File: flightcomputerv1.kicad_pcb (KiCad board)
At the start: 2 copper layers, 190.5 x 101.6 mm, 3 parts, among them U1 Teensy4.1, U2 MS5607-02BA, U3 BMI088

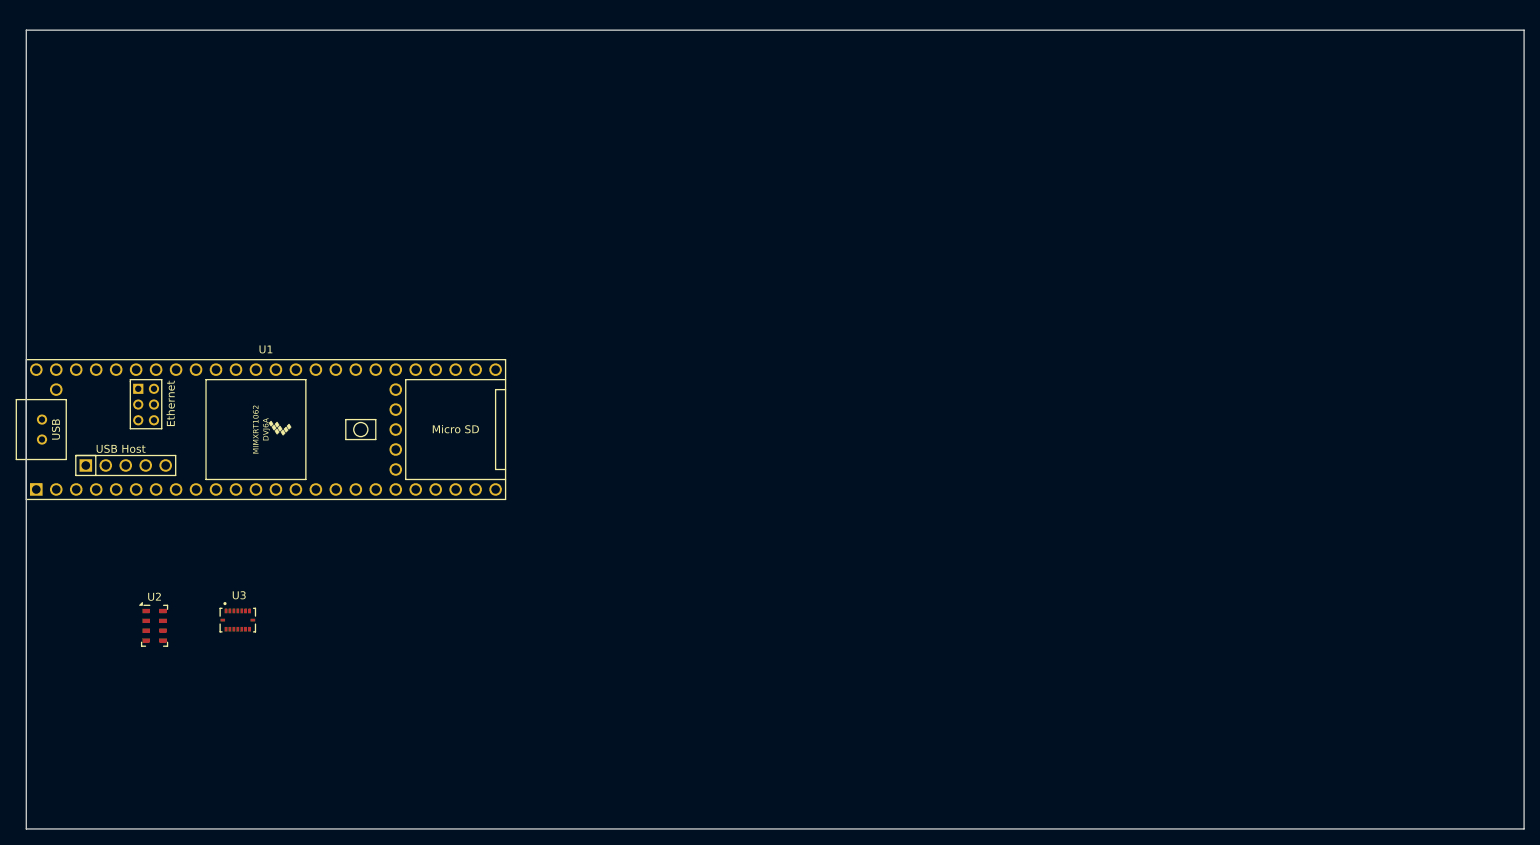
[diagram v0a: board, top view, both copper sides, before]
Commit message: started placement
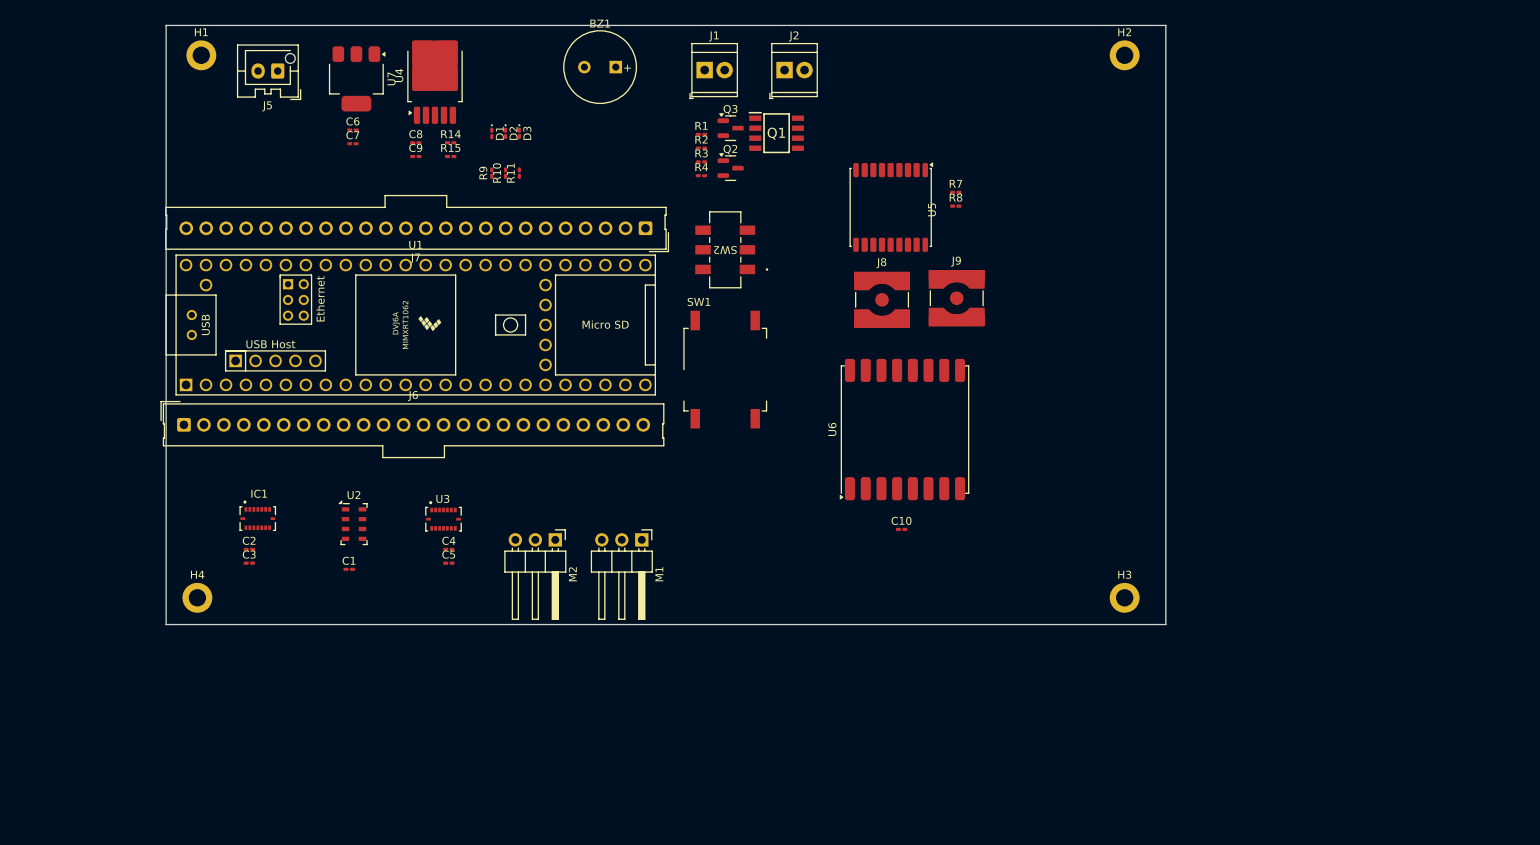
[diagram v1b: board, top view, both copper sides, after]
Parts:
- added BZ1: Buzzer, Buzzer_Beeper:MagneticBuzzer_PUI_AT-0927-TT-6-R, F.Cu at (108.0, 55.5)
- added C1: 0.1uF, Capacitor_SMD:C_0201_0603Metric_Pad0.64x0.40mm_HandSolder, F.Cu at (74.1, 119.4)
- added C10: 10uF, Capacitor_SMD:C_0201_0603Metric_Pad0.64x0.40mm_HandSolder, F.Cu at (144.3, 114.3)
- added C2: 1uF, Capacitor_SMD:C_0201_0603Metric_Pad0.64x0.40mm_HandSolder, F.Cu at (61.4, 116.8)
- added C3: 10uF, Capacitor_SMD:C_0201_0603Metric_Pad0.64x0.40mm_HandSolder, F.Cu at (61.4, 118.6)
- added C4: 0.1uF, Capacitor_SMD:C_0201_0603Metric_Pad0.64x0.40mm_HandSolder, F.Cu at (86.8, 116.8)
- added C5: 0.1uF, Capacitor_SMD:C_0201_0603Metric_Pad0.64x0.40mm_HandSolder, F.Cu at (86.8, 118.6)
- added C6: 100nF, Capacitor_SMD:C_0201_0603Metric_Pad0.64x0.40mm_HandSolder, F.Cu at (74.6, 63.5)
- added C7: 10uF, Capacitor_SMD:C_0201_0603Metric_Pad0.64x0.40mm_HandSolder, F.Cu at (74.6, 65.2)
- added C8: 10uF, Capacitor_SMD:C_0201_0603Metric_Pad0.64x0.40mm_HandSolder, F.Cu at (82.6, 65.1)
- added C9: 22uF, Capacitor_SMD:C_0201_0603Metric_Pad0.64x0.40mm_HandSolder, F.Cu at (82.6, 66.9)
- added D1: LED, LED_SMD:LED_0201_0603Metric_Pad0.64x0.40mm_HandSolder, F.Cu at (92.2, 63.9)
- added D2: LED, LED_SMD:LED_0201_0603Metric_Pad0.64x0.40mm_HandSolder, F.Cu at (94.0, 63.9)
- added D3: LED, LED_SMD:LED_0201_0603Metric_Pad0.64x0.40mm_HandSolder, F.Cu at (95.7, 63.9)
- added H1: MountingHole_Pad, MountingHole:MountingHole_2.2mm_M2_DIN965_Pad, F.Cu at (55.3, 54.0)
- added H2: MountingHole_Pad, MountingHole:MountingHole_2.2mm_M2_DIN965_Pad, F.Cu at (172.7, 54.0)
- added H3: MountingHole_Pad, MountingHole:MountingHole_2.2mm_M2_DIN965_Pad, F.Cu at (172.7, 123.0)
- added H4: MountingHole_Pad, MountingHole:MountingHole_2.2mm_M2_DIN965_Pad, F.Cu at (54.8, 123.0)
- added IC1: MMC5983MA, HPRfootprints:PQFN50P450X300X100-16N, F.Cu at (62.5, 112.9)
- added J1: Screw_Terminal_01x02, TerminalBlock_TE-Connectivity:TerminalBlock_TE_282834-2_1x02_P2.54mm_Horizontal, F.Cu at (119.3, 55.9)
- added J2: Screw_Terminal_01x02, TerminalBlock_TE-Connectivity:TerminalBlock_TE_282834-2_1x02_P2.54mm_Horizontal, F.Cu at (129.5, 55.9)
- added J5: Conn_01x02, Connector_JST:JST_XA_B02B-XASK-1-A_1x02_P2.50mm_Vertical, F.Cu at (65.0, 56.0)
- added J6: Conn_01x24, Connector_Molex:Molex_SL_171971-0024_1x24_P2.54mm_Vertical, F.Cu at (53.1, 101.0)
- added J7: Conn_01x24, Connector_Molex:Molex_SL_171971-0024_1x24_P2.54mm_Vertical, F.Cu at (111.8, 76.0)
- added J8: Conn_Coaxial, Connector_Coaxial:SMA_Amphenol_132134-10_Vertical, F.Cu at (141.9, 85.1)
- added J9: Conn_Coaxial, Connector_Coaxial:SMA_Amphenol_132134-10_Vertical, F.Cu at (151.4, 84.9)
- added M1: Motor_Servo, Connector_PinHeader_2.54mm:PinHeader_1x03_P2.54mm_Horizontal, F.Cu at (111.3, 115.6)
- added M2: Motor_Servo, Connector_PinHeader_2.54mm:PinHeader_1x03_P2.54mm_Horizontal, F.Cu at (100.3, 115.6)
- added Q1: SI4925DDY-T1-GE3, HPRfootprints:SOIC127P600X175-8N, F.Cu at (128.4, 63.9)
- added Q2: MMBT3904, Package_TO_SOT_SMD:SOT-23, F.Cu at (122.6, 68.3)
- added Q3: MMBT3904, Package_TO_SOT_SMD:SOT-23, F.Cu at (122.6, 63.3)
- added R1: 10K, Resistor_SMD:R_0201_0603Metric_Pad0.64x0.40mm_HandSolder, F.Cu at (118.9, 64.1)
- added R10: 150, Resistor_SMD:R_0201_0603Metric_Pad0.64x0.40mm_HandSolder, F.Cu at (94.0, 69.0)
- added R11: 150, Resistor_SMD:R_0201_0603Metric_Pad0.64x0.40mm_HandSolder, F.Cu at (95.7, 69.0)
- added R14: 1.2k, Resistor_SMD:R_0201_0603Metric_Pad0.64x0.40mm_HandSolder, F.Cu at (87.0, 65.1)
- added R15: 4.7k, Resistor_SMD:R_0201_0603Metric_Pad0.64x0.40mm_HandSolder, F.Cu at (87.0, 66.9)
- added R2: 1K, Resistor_SMD:R_0201_0603Metric_Pad0.64x0.40mm_HandSolder, F.Cu at (118.9, 65.8)
- added R3: 10K, Resistor_SMD:R_0201_0603Metric_Pad0.64x0.40mm_HandSolder, F.Cu at (118.9, 67.6)
- added R4: 1K, Resistor_SMD:R_0201_0603Metric_Pad0.64x0.40mm_HandSolder, F.Cu at (118.9, 69.3)
- added R7: 4.7k, Resistor_SMD:R_0201_0603Metric_Pad0.64x0.40mm_HandSolder, F.Cu at (151.2, 71.4)
- added R8: 4.7k, Resistor_SMD:R_0201_0603Metric_Pad0.64x0.40mm_HandSolder, F.Cu at (151.2, 73.2)
- added R9: 150, Resistor_SMD:R_0201_0603Metric_Pad0.64x0.40mm_HandSolder, F.Cu at (92.2, 69.0)
- added SW1: SW_MEC_5G, Button_Switch_SMD:SW_MEC_5GSH9, F.Cu at (121.9, 94.0)
- added SW2: SLW-913535-2A-SMT, HPRfootprints:SLW-913535_CUD, F.Cu at (121.9, 78.7)
- added U4: MIC29302AWD, Package_TO_SOT_SMD:TO-252-5_TabPin3, F.Cu at (85.0, 56.6)
- added U5: MAX-M10S, RF_GPS:ublox_MAX, F.Cu at (143.0, 73.3)
- added U6: RFM95W-915S2, RF_Module:HOPERF_RFM9XW_SMD, F.Cu at (144.8, 101.6)
- added U7: LD1117S50TR_SOT223, Package_TO_SOT_SMD:SOT-223-3_TabPin2, F.Cu at (75.0, 57.0)
- U1: footprint teensy:Teensy41 -> HPRfootprints:Teensy41
- U3: footprint BMI088:PQFN50P450X300X100-16N -> HPRfootprints:PQFN50P450X300X100-16N
- moved U3 29.1 mm to (86.1, 113.0)
- moved U2 28.5 mm to (74.7, 113.6)
- moved U1 23.2 mm to (82.5, 88.3)
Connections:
- U1 pad 1: unconnected-(U1-GND-Pad1) -> GND
- U1 pad 10: unconnected-(U1-8_TX2_IN1-Pad10) -> /FREE1
- U1 pad 11: unconnected-(U1-9_OUT1C-Pad11) -> /FREE2
- U1 pad 12: unconnected-(U1-10_CS_MQSR-Pad12) -> /baro_cs
- U1 pad 13: unconnected-(U1-11_MOSI_CTX1-Pad13) -> /SENSE_mosi
- U1 pad 14: unconnected-(U1-12_MISO_MQSL-Pad14) -> /SENSE_miso
- U1 pad 15: unconnected-(U1-3V3-Pad15) -> /teensy_3.3v
- U1 pad 16: unconnected-(U1-24_A10_TX6_SCL2-Pad16) -> /FREE3
- U1 pad 17: unconnected-(U1-25_A11_RX6_SDA2-Pad17) -> /FREE4
- U1 pad 18: unconnected-(U1-26_A12_MOSI1-Pad18) -> /radio_mosi
- U1 pad 19: unconnected-(U1-27_A13_SCK1-Pad19) -> /radio_sck
- U1 pad 2: unconnected-(U1-0_RX1_CRX2_CS1-Pad2) -> /radio_reset
- U1 pad 20: unconnected-(U1-28_RX7-Pad20) -> /servo2_pwm
- U1 pad 21: unconnected-(U1-29_TX7-Pad21) -> /servo1_pwm
- U1 pad 22: unconnected-(U1-30_CRX3-Pad22) -> /FREE5
- U1 pad 23: unconnected-(U1-31_CTX3-Pad23) -> /FREE6
- U1 pad 24: unconnected-(U1-32_OUT1B-Pad24) -> /radio_cs
- U1 pad 25: unconnected-(U1-33_MCLK2-Pad25) -> /buzz_pwm
- U1 pad 26: unconnected-(U1-34_RX8-Pad26) -> /PYRO1
- U1 pad 27: unconnected-(U1-35_TX8-Pad27) -> /PYRO2
- U1 pad 28: unconnected-(U1-36_CS-Pad28) -> /imu_gyro_cs
- U1 pad 29: unconnected-(U1-37_CS-Pad29) -> /imu_accel_cs
- U1 pad 3: unconnected-(U1-1_TX1_CTX2_MISO1-Pad3) -> /radio_miso
- U1 pad 30: unconnected-(U1-38_CS1_IN1-Pad30) -> /mag_cs
- U1 pad 31: unconnected-(U1-39_MISO1_OUT1A-Pad31) -> /LED3
- U1 pad 32: unconnected-(U1-40_A16-Pad32) -> /LED2
- U1 pad 33: unconnected-(U1-41_A17-Pad33) -> /LED1
- U1 pad 34: unconnected-(U1-GND-Pad34) -> GND
- U1 pad 35: unconnected-(U1-13_SCK_LED-Pad35) -> /SENSE_sck
- U1 pad 36: unconnected-(U1-14_A0_TX3_SPDIF_OUT-Pad36) -> /FREE12
- U1 pad 37: unconnected-(U1-15_A1_RX3_SPDIF_IN-Pad37) -> /FREE11
- U1 pad 38: unconnected-(U1-16_A2_RX4_SCL1-Pad38) -> /FREE10
- U1 pad 39: unconnected-(U1-17_A3_TX4_SDA1-Pad39) -> /FREE9
- U1 pad 4: unconnected-(U1-2_OUT2-Pad4) -> /radio_dio5
- U1 pad 40: unconnected-(U1-18_A4_SDA-Pad40) -> /GPS_sda
- U1 pad 41: unconnected-(U1-19_A5_SCL-Pad41) -> /GPS_scl
- U1 pad 42: unconnected-(U1-20_A6_TX5_LRCLK1-Pad42) -> /GPS_reset
- U1 pad 43: unconnected-(U1-21_A7_RX5_BCLK1-Pad43) -> /GPS_int
- U1 pad 44: unconnected-(U1-22_A8_CTX1-Pad44) -> /FREE8
- U1 pad 45: unconnected-(U1-23_A9_CRX1_MCLK1-Pad45) -> /FREE7
- U1 pad 46: unconnected-(U1-3V3-Pad46) -> /teensy_3.3v
- U1 pad 47: unconnected-(U1-GND-Pad47) -> GND
- U1 pad 48: unconnected-(U1-VIN-Pad48) -> /ldo_5v
- U1 pad 5: unconnected-(U1-3_LRCLK2-Pad5) -> /radio_dio4
- U1 pad 51: unconnected-(U1-3V3-Pad51) -> /teensy_3.3v
- U1 pad 52: unconnected-(U1-GND-Pad52) -> GND
- U1 pad 53: unconnected-(U1-PROGRAM-Pad53) -> Net-(U1-PROGRAM)
- U1 pad 54: unconnected-(U1-ON_OFF-Pad54) -> /teensy_onoff
- U1 pad 6: unconnected-(U1-4_BCLK2-Pad6) -> /radio_dio3
- U1 pad 7: unconnected-(U1-5_IN2-Pad7) -> /radio_dio2
- U1 pad 8: unconnected-(U1-6_OUT1D-Pad8) -> /radio_dio1
- U1 pad 9: unconnected-(U1-7_RX2_OUT1A-Pad9) -> /radio_dio0
- U2 pad 1: unconnected-(U2-VDD-Pad1) -> /teensy_3.3v
- U2 pad 2: unconnected-(U2-PS-Pad2) -> GND
- U2 pad 3: unconnected-(U2-GND-Pad3) -> GND
- U2 pad 4: Net-(U2-CSB-Pad4) -> /baro_cs
- U2 pad 5: Net-(U2-CSB-Pad4) -> /baro_cs
- U2 pad 6: unconnected-(U2-SDO-Pad6) -> /SENSE_miso
- U2 pad 7: unconnected-(U2-SDI/SDA-Pad7) -> /SENSE_mosi
- U2 pad 8: unconnected-(U2-SCLK-Pad8) -> /SENSE_sck
- U3 pad 10: unconnected-(U3-SDO2-Pad10) -> /SENSE_miso
- U3 pad 11: unconnected-(U3-VDDIO-Pad11) -> /teensy_3.3v
- U3 pad 12: unconnected-(U3-INT3-Pad12) -> /imu_gyro_int1
- U3 pad 14: unconnected-(U3-CSB1-Pad14) -> /imu_accel_cs
- U3 pad 15: unconnected-(U3-SDO1-Pad15) -> /SENSE_miso
- U3 pad 16: unconnected-(U3-INT1-Pad16) -> /imu_accel_int1
- U3 pad 2: unconnected-(U3-NC-Pad2) -> GND
- U3 pad 3: unconnected-(U3-VDD-Pad3) -> /teensy_3.3v
- U3 pad 4: unconnected-(U3-GNDA-Pad4) -> GND
- U3 pad 5: unconnected-(U3-CSB2-Pad5) -> /imu_gyro_cs
- U3 pad 6: unconnected-(U3-GNDIO-Pad6) -> GND
- U3 pad 7: unconnected-(U3-PS-Pad7) -> GND
- U3 pad 8: unconnected-(U3-SCL/SCK-Pad8) -> /SENSE_sck
- U3 pad 9: unconnected-(U3-SDA/SDI-Pad9) -> /SENSE_mosi
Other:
- board size 190.5 x 101.6 mm -> 127.2 x 76.2 mm
